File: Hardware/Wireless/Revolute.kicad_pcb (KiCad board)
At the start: 4 copper layers, 19.8 x 20 mm, 60 parts, among them U1 BQ27441-G1, U10 Button, U2 nrf52833_qfn40, U3 AS5600, U4 AP2112K-3.3, U5 BQ24075RGT, U6 Button, U8 Button, U9 Button, X1 32.768 kHz, X2 32MHZ

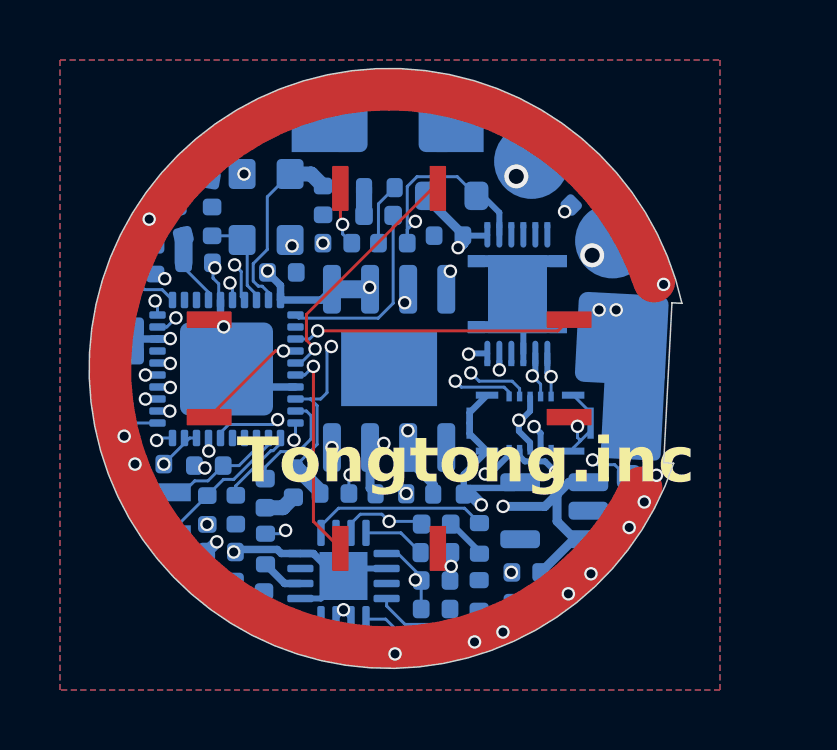
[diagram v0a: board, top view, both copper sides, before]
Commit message: new gerbers
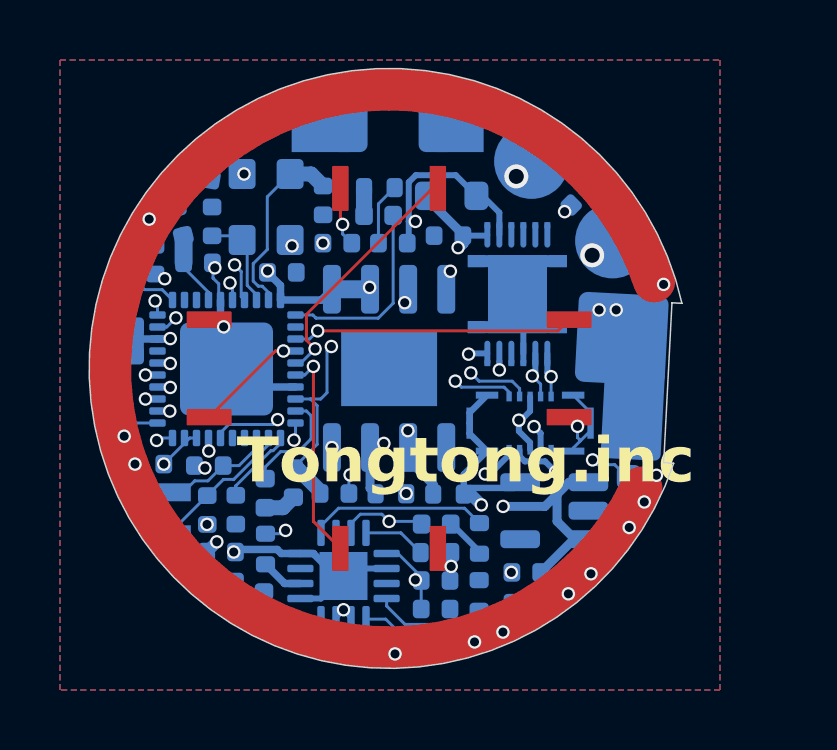
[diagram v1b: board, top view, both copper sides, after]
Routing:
- net Batteryin: track 22.0 -> 21.5 mm
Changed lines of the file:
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@@
   (segment (start 171.895 102.07) (end 171.875 102.05) (width 0.1) (layer "B.Cu") (net 3))
   (segment (start 175.325 96.825) (end 175.325 97.095) (width 0.2) (layer "B.Cu") (net 3))
-  (segment (start 167.985 93.325) (end 170.639264 93.325) (width 0.1) (layer "B.Cu") (net 4))
-  (segment (start 167.88 93.22) (end 167.985 93.325) (width 0.1) (layer "B.Cu") (net 4))
   (segment (start 171.135 92.829264) (end 171.135 89.9) (width 0.1) (layer "B.Cu") (net 4))
+  (segment (start 167.88 93.22) (end 168.46 93.22) (width 0.1) (layer "B.Cu") (net 4))
   (segment (start 170.639264 93.325) (end 171.135 92.829264) (width 0.1) (layer "B.Cu") (net 4))
+  (segment (start 168.565 93.325) (end 170.639264 93.325) (width 0.1) (layer "B.Cu") (net 4))
+  (segment (start 168.46 93.22) (end 168.565 93.325) (width 0.1) (layer "B.Cu") (net 4))
   (segment (start 170.165 89.9) (end 170.165 88.975) (width 0.54) (layer "B.Cu") (net 5))
   (via (at 163.199979 92.750054) (size 0.45) (drill 0.3) (layers "F.Cu" "B.Cu") (net 6))
@@
   (segment (start 173.9 90.1) (end 174.73 89.27) (width 0.4) (layer "In2.Cu") (net 11))
   (segment (start 174.675 89.806579) (end 174.675 90.55) (width 0.2) (layer "B.Cu") (net 11))
-  (segment (start 171.605 90.825) (end 171.605 90.37) (width 0.1) (layer "B.Cu") (net 11))
-  (segment (start 171.929739 88.61) (end 173.27383 88.61) (width 0.1) (layer "B.Cu") (net 11))
-  (segment (start 171.605 90.825) (end 171.605 88.934739) (width 0.1) (layer "B.Cu") (net 11))
+  (segment (start 173.22383 88.56) (end 173.911772 89.247942) (width 0.2) (layer "B.Cu") (net 11))
+  (segment (start 171.655 88.795) (end 171.89 88.56) (width 0.2) (layer "B.Cu") (net 11))
+  (segment (start 171.605 90.825) (end 171.655 90.775) (width 0.2) (layer "B.Cu") (net 11))
   (segment (start 178.716087 94.711271) (end 178.716087 93.646926) (width 0.2) (layer "B.Cu") (net 11))
   (segment (start 178.57 93.05) (end 178.716087 93.196087) (width 0.2) (layer "B.Cu") (net 11))
+  (segment (start 171.875 90.1) (end 171.655 90.1) (width 0.2) (layer "B.Cu") (net 11))
   (segment (start 178.716087 93.646926) (end 179.171757 93.191256) (width 0.2) (layer "B.Cu") (net 11))
   (segment (start 174.116363 89.247942) (end 174.675 89.806579) (width 0.2) (layer "B.Cu") (net 11))
@@
   (segment (start 178.716087 93.766087) (end 178 93.05) (width 0.2) (layer "B.Cu") (net 11))
   (segment (start 174.275 94.5) (end 173.675 94.5) (width 0.2) (layer "B.Cu") (net 11))
-  (segment (start 173.27383 88.61) (end 173.911772 89.247942) (width 0.1) (layer "B.Cu") (net 11))
+  (segment (start 171.655 90.1) (end 171.655 88.795) (width 0.2) (layer "B.Cu") (net 11))
   (segment (start 173.675 94.5) (end 173.65 94.525) (width 0.2) (layer "B.Cu") (net 11))
+  (segment (start 171.89 88.56) (end 173.22383 88.56) (width 0.2) (layer "B.Cu") (net 11))
   (segment (start 178.716087 94.711271) (end 178.716087 93.766087) (width 0.2) (layer "B.Cu") (net 11))
+  (segment (start 171.655 90.775) (end 171.655 90.1) (width 0.2) (layer "B.Cu") (net 11))
   (segment (start 178.716087 93.196087) (end 178.716087 94.711271) (width 0.2) (layer "B.Cu") (net 11))
-  (segment (start 171.605 90.37) (end 171.875 90.1) (width 0.1) (layer "B.Cu") (net 11))
   (segment (start 178 93.05) (end 178 93) (width 0.2) (layer "B.Cu") (net 11))
-  (segment (start 171.605 88.934739) (end 171.929739 88.61) (width 0.1) (layer "B.Cu") (net 11))
   (segment (start 173.055 100.19) (end 173.095805 100.19) (width 0.2) (layer "B.Cu") (net 12))
   (segment (start 174.011227 101.105422) (end 174.011227 101.176601) (width 0.2) (layer "B.Cu") (net 12))
